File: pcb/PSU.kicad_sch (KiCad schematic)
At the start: 26 parts

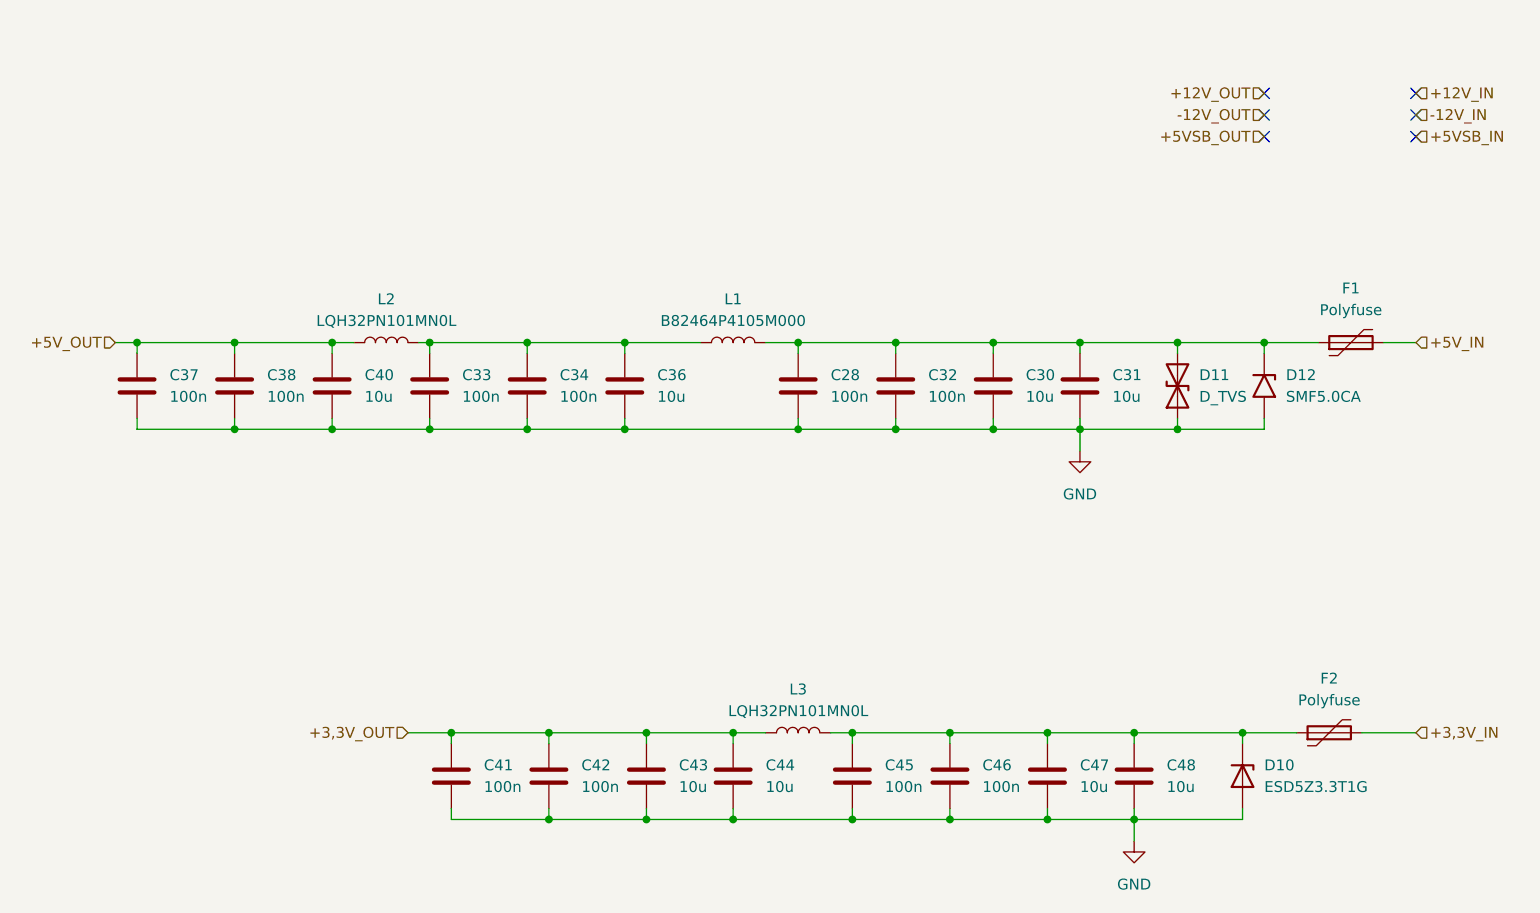
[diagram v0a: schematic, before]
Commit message: New power design
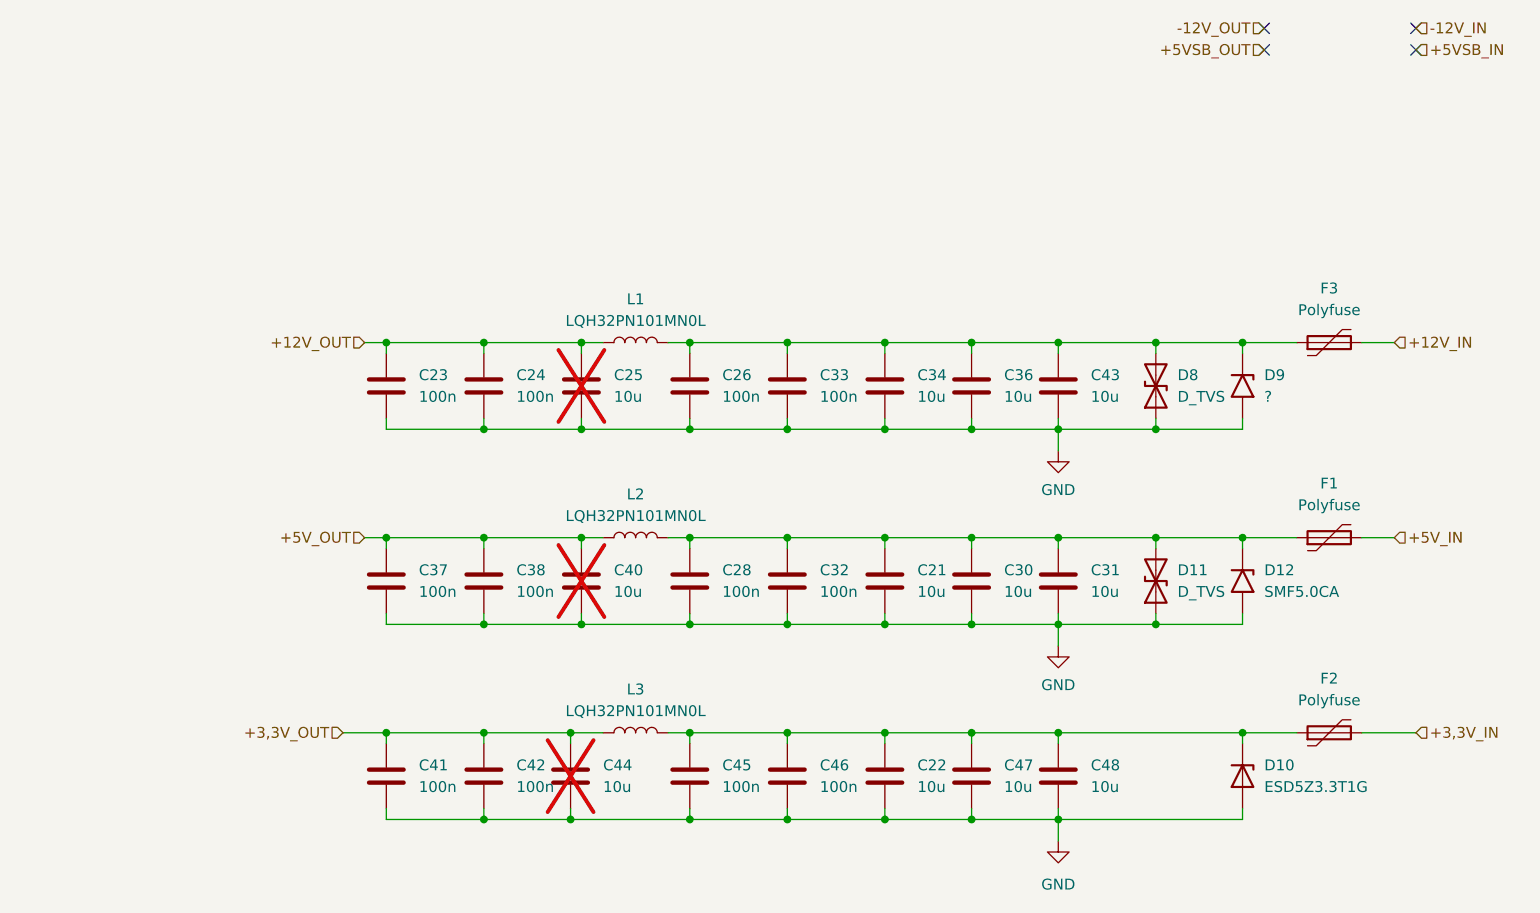
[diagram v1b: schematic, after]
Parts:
- added C21, C22, C25: 10u, Capacitor_SMD:C_1206_3216Metric_Pad1.33x1.80mm_HandSolder, symbol Device:C
- added C23, C24, C26: 100n, Capacitor_SMD:C_0603_1608Metric_Pad1.08x0.95mm_HandSolder, symbol Device:C
- added D8: D_TVS, Diode_SMD:D_MiniMELF, symbol Device:D_TVS
- added D9: ?, Diode_SMD:D_SMF, symbol Diode:SMF5V0A
- added F3: Polyfuse, Fuse:Fuse_1206_3216Metric_Pad1.42x1.75mm_HandSolder, symbol Device:Polyfuse
- C34: value 100n -> 10u; footprint Capacitor_SMD:C_0603_1608Metric_Pad1.08x0.95mm_HandSolder -> Capacitor_SMD:C_1206_3216Metric_Pad1.33x1.80mm_HandSolder
- C40, C44: now not fitted; now left out of the parts list
- L1: value B82464P4105M000 -> LQH32PN101MN0L; footprint Inductor_SMD:L_10.4x10.4_H4.8 -> Inductor_SMD:L_1210_3225Metric
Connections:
- net +12V_IN: now also F3.2
- net +12V_OUT: now also L1.1, C23.1, C24.1, C25.1
- net +3,3V_OUT: no longer C43.1
- net GND: now also C21.2, C22.2, C23.2, C24.2, C25.2, C26.2, D8.1 (A1), D9.2 (A2)
- net at C45.1, C46.1, C47.1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: now also C22.1
- net at C28.1, C30.1, C31.1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: now also L2.2, C21.1; no longer L1.2
- net at C33.1, C34.1, C36.1: now also C43.1, L1.2, C26.1, D8.2 (A2), D9.1 (A1), F3.1; no longer L1.1, L2.2
- no-connect marks 6 -> 4
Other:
- moved on the sheet: C28, C30, C31, C32, C37, C38, C41, C42, C45, C46, C47, C48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
